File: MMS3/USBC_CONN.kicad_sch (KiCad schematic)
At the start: 5 parts, among them J800 USB_C_Receptacle_USB2.0_16P, U401 TPD2EUSB30DRTR-TP

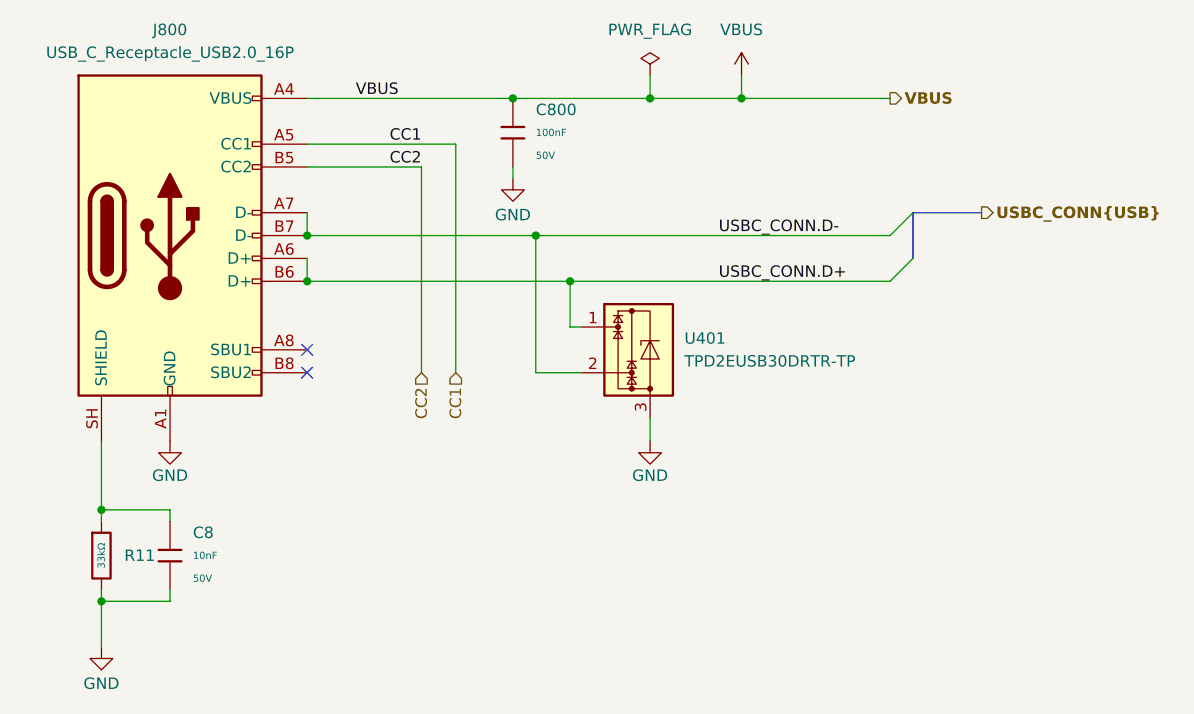
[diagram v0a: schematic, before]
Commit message: backup commit
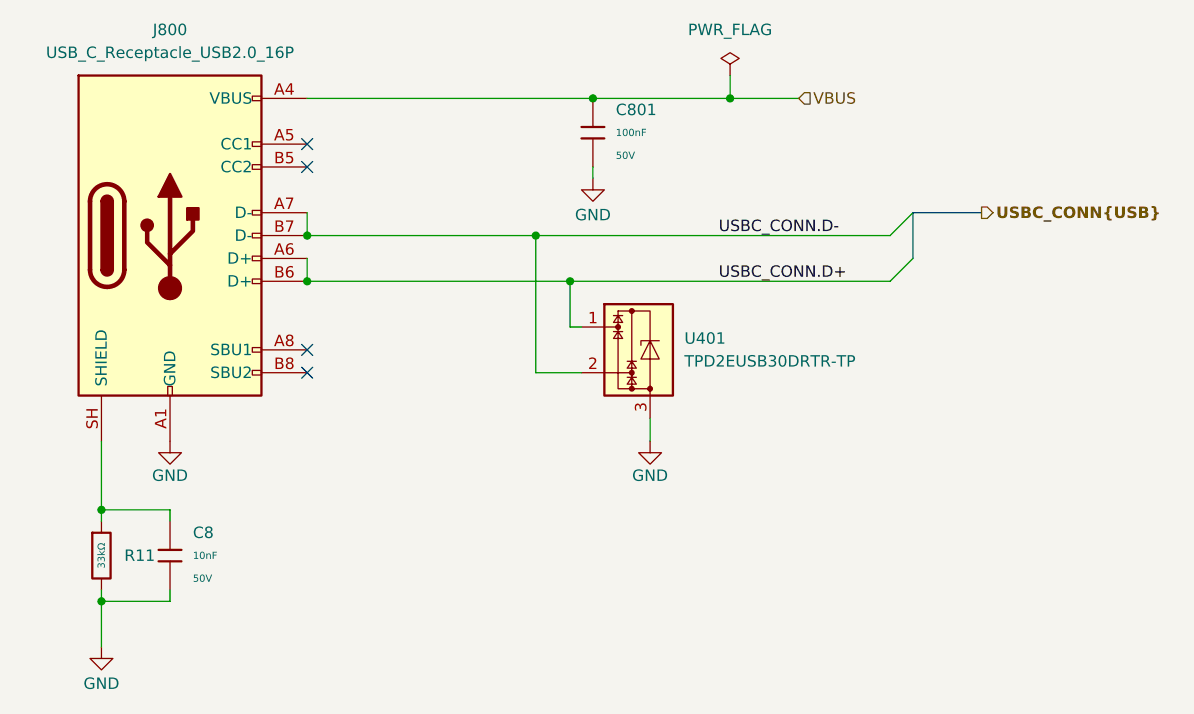
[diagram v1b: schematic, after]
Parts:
- removed C800: 100nF, PCM_JLCPCB:C_0402, symbol PCM_JLCPCB-Capacitors:0402,100nF,(2)
- added C801: 100nF, PCM_JLCPCB:C_0402, symbol PCM_JLCPCB-Capacitors:0402,100nF,(2)
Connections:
- net GND: now also C801.2
- net VBUS: now also C801.1
- net CC1: no longer names the net of J800.A5 (CC1)
- net CC2: no longer names the net of J800.B5 (CC2)
- no-connect marks 2 -> 4
